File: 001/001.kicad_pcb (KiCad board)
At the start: 2 copper layers, 76.2 x 78.7 mm, 5 parts, among them SW1 SW_SPDT, U1 MF-Jalisco

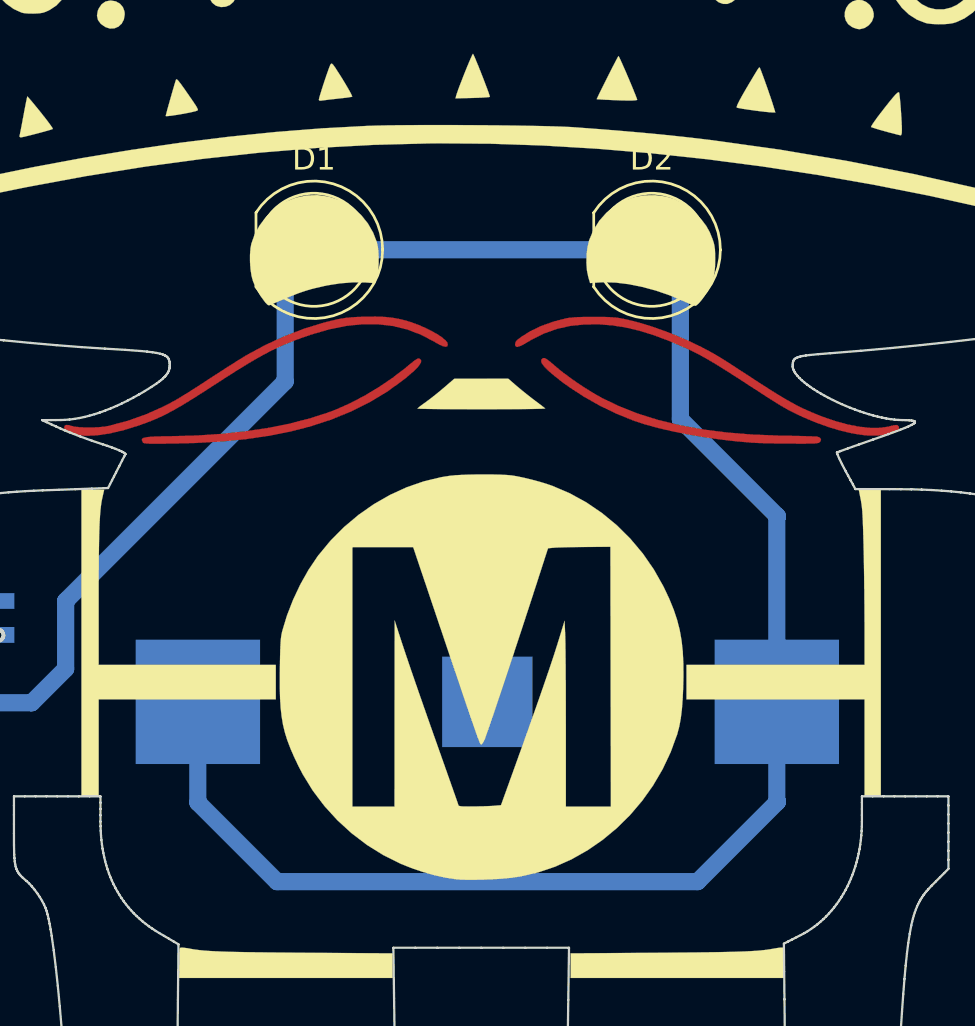
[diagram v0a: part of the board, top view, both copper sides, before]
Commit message: Add Battery Holder WA-BCMC and Straw Hat Led
Add Battery Holder WA-BCMC and Straw Hat Led
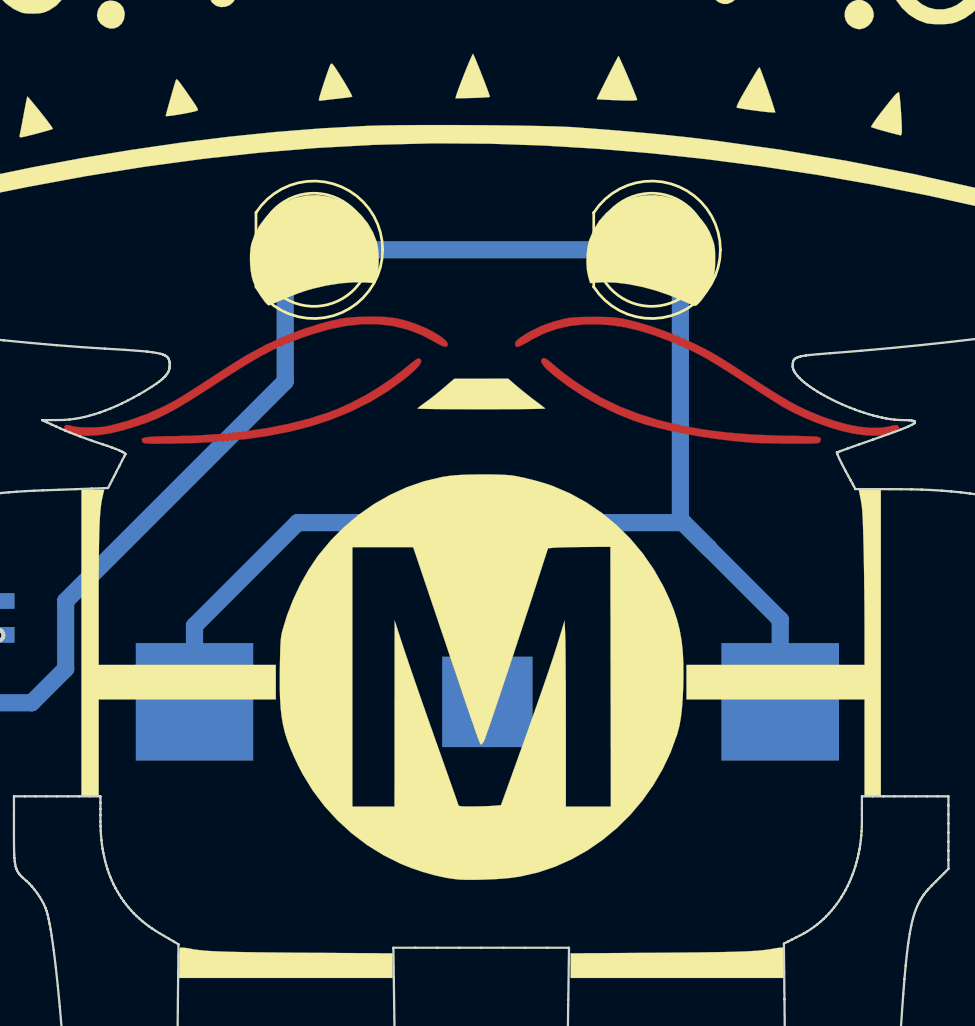
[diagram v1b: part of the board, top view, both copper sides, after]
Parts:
- BT1: footprint 001:S8211R -> 001:WA-BCMC
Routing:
- net +3V3: track 59.2 -> 50.3 mm
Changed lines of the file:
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@@
-(kicad_pcb (version 20171130) (host pcbnew 5.1.3-ffb9f22~84~ubuntu18.04.1)
+(kicad_pcb (version 20171130) (host pcbnew 5.1.4-e60b266~84~ubuntu18.04.1)
   (general
     (thickness 1.6002)
     (drawings 0)
-    (tracks 17)
+    (tracks 15)
     (zones 0)
     (modules 5)
@@
     (descr "LED, Round, FlatTop, diameter 5.0mm, 2 pins, http://www.kingbright.com/attachments/file/psearch/000/00/00/L-483GDT(Ver.15B).pdf")
     (tags "LED Round FlatTop diameter 5.0mm 2 pins")
-    (fp_text reference D1 (at 1.27 -4.01) (layer F.SilkS)
+    (fp_text reference D1 (at 1.27 -4.01) (layer F.Fab)
       (effects (font (size 1 1) (thickness 0.15)))
     )
@@
     (pad 2 thru_hole circle (at 2.54 0) (size 1.8 1.8) (drill 0.9) (layers *.Cu *.Mask)
       (net 1 "Net-(D1-Pad2)"))
-    (model ${KISYS3DMOD}/LED_THT.3dshapes/LED_D5.0mm_FlatTop.wrl
-      (at (xyz 0 0 0))
-      (scale (xyz 1 1 1))
-      (rotate (xyz 0 0 0))
+    (model "${KISYS3DMOD}/LED_THT.3dshapes/8mm 0.5w straw hat.STEP"
+      (offset (xyz 1.3 0 2.9))
+      (scale (xyz 0.5 0.7 0.5))
+      (rotate (xyz -90 0 180))
     )
   )
@@
     (descr "LED, Round, FlatTop, diameter 5.0mm, 2 pins, http://www.kingbright.com/attachments/file/psearch/000/00/00/L-483GDT(Ver.15B).pdf")
     (tags "LED Round FlatTop diameter 5.0mm 2 pins")
-    (fp_text reference D2 (at 1.27 -4.01) (layer F.SilkS)
+    (fp_text reference D2 (at 1.27 -4.01) (layer F.Fab)
       (effects (font (size 1 1) (thickness 0.15)))
     )
@@
     (pad 1 thru_hole rect (at 0 0) (size 1.8 1.8) (drill 0.9) (layers *.Cu *.Mask)
       (net 1 "Net-(D1-Pad2)"))
-    (model ${KISYS3DMOD}/LED_THT.3dshapes/LED_D5.0mm_FlatTop.wrl
-      (at (xyz 0 0 0))
-      (scale (xyz 1 1 1))
-      (rotate (xyz 0 0 0))
-    )
-  )
-  (module 001:S8211R (layer Back)
-    (at 137.3886 105.7148)
-    (fp_text reference BT1 (at 10.16 -12.446) (layer B.SilkS)
-      (effects (font (size 1 1) (thickness 0.15)) (justify mirror))
-    )
-    (fp_text value Battery_3V_Coin (at -9.398 10.16) (layer B.Fab)
-      (effects (font (size 1 1) (thickness 0.15)) (justify mirror))
-    )
-    (fp_line (start 12.8 9.1) (end 12.8 -10.9) (layer B.SilkS) (width 0.15))
-    (fp_line (start -12.8 9.1) (end 12.8 9.1) (layer B.SilkS) (width 0.15))
-    (fp_line (start -12.8 -10.9) (end -12.8 9.1) (layer B.SilkS) (width 0.15))
-    (fp_line (start 12.8 -10.9) (end -12.8 -10.9) (layer B.SilkS) (width 0.15))
-    (pad 1 smd rect (at 12.8 0) (size 5.5 5.5) (layers Back B.Paste B.Mask)
-      (net 2 +3V3))
-    (pad 1 smd rect (at -12.8 0) (size 5.5 5.5) (layers Back B.Paste B.Mask)
-      (net 2 +3V3))
-    (pad 2 smd rect (at 0 0) (size 4 4) (layers Back B.Paste B.Mask)
-      (net 3 GND))
-    (model /home/greynaga/Desktop/kicad/packages3d/Battery.3dshapes/s8211-46r.stp
-      (offset (xyz 0 6 4))
-      (scale (xyz 1 1 1))
-      (rotate (xyz 0 90 -90))
-    )
-    (model /home/greynaga/Desktop/kicad/packages3d/Battery.3dshapes/CR-2032-01.step
-      (offset (xyz 0 0 3))
-      (scale (xyz 1 1 1))
-      (rotate (xyz 90 0 0))
+    (model "${KISYS3DMOD}/LED_THT.3dshapes/8mm 0.5w straw hat.STEP"
+      (offset (xyz 1.3 0 2.9))
+      (scale (xyz 0.5 0.7 0.5))
+      (rotate (xyz -90 0 180))
     )
   )
@@
     )
   )
-  (via (at 115.7351 102.77094) (size 0.6858) (drill 0.3302) (layers Front Back) (net 3))
+  (module 001:WA-BCMC (layer Back)
+    (at 137.3886 105.7148)
+    (fp_text reference BT1 (at 10.16 -12.446) (layer B.Fab)
+      (effects (font (size 1 1) (thickness 0.15)) (justify mirror))
+    )
+    (fp_text value Battery_3V_Coin (at -9.398 10.16) (layer B.Fab)
+      (effects (font (size 1 1) (thickness 0.15)) (justify mirror))
+    )
+    (fp_line (start 12.8 -10.9) (end -12.8 -10.9) (layer B.Fab) (width 0.15))
+    (fp_line (start -12.8 -10.9) (end -12.8 9.1) (layer B.Fab) (width 0.15))
+    (fp_line (start -12.8 9.1) (end 12.8 9.1) (layer B.Fab) (width 0.15))
+    (fp_line (start 12.8 9.1) (end 12.8 -10.9) (layer B.Fab) (width 0.15))
+    (pad 2 smd rect (at 0 0) (size 4 4) (layers Back B.Paste B.Mask)
+      (net 3 GND))
+    (pad 1 smd rect (at -12.95 0) (size 5.2 5.2) (layers Back B.Paste B.Mask)
+      (net 2 +3V3))
+    (pad 1 smd rect (at 12.95 0) (size 5.2 5.2) (layers Back B.Paste B.Mask)
+      (net 2 +3V3))
+    (model ${KISYS3DMOD}/Battery.3dshapes/s8211-46r.stp
+      (offset (xyz 0 -6 4.1))
+      (scale (xyz 1 1 1))
+      (rotate (xyz 0 90 90))
+    )
+  )
   (segment (start 130.9878 85.725) (end 143.383 85.725) (width 0.762) (layer Back) (net 1))
-  (segment (start 145.923 93.218) (end 145.923 85.725) (width 0.762) (layer Back) (net 2))
-  (segment (start 150.214 97.509) (end 145.923 93.218) (width 0.762) (layer Back) (net 2))
-  (segment (start 150.1886 97.5344) (end 150.1886 105.7148) (width 0.762) (layer Back) (net 2))
-  (segment (start 150.214 97.509) (end 150.1886 97.5344) (width 0.762) (layer Back) (net 2))
-  (segment (start 124.5886 110.1666) (end 124.5886 105.7148) (width 0.762) (layer Back) (net 2))
-  (segment (start 128.087 113.665) (end 124.5886 110.1666) (width 0.762) (layer Back) (net 2))
-  (segment (start 150.214 110.136) (end 146.685 113.665) (width 0.762) (layer Back) (net 2))
-  (segment (start 146.685 113.665) (end 128.087 113.665) (width 0.762) (layer Back) (net 2))
-  (segment (start 150.1886 110.1106) (end 150.1886 105.7148) (width 0.762) (layer Back) (net 2))
-  (segment (start 150.214 110.136) (end 150.1886 110.1106) (width 0.762) (layer Back) (net 2))
+  (segment (start 150.3386 102.0786) (end 150.3386 105.7148) (width 0.762) (layer Back) (net 2))
+  (segment (start 147.193 98.933) (end 150.3386 102.0786) (width 0.762) (layer Back) (net 2))
+  (segment (start 145.923 97.663) (end 147.193 98.933) (width 0.762) (layer Back) (net 2))
+  (segment (start 145.923 85.725) (end 145.923 97.663) (width 0.762) (layer Back) (net 2))
+  (segment (start 146.05 97.79) (end 147.193 98.933) (width 0.762) (layer Back) (net 2))
+  (segment (start 129.0014 97.79) (end 146.05 97.79) (width 0.762) (layer Back) (net 2))
+  (segment (start 124.4386 105.7148) (end 124.4386 102.3528) (width 0.762) (layer Back) (net 2))
+  (segment (start 124.4386 102.3528) (end 129.0014 97.79) (width 0.762) (layer Back) (net 2))
+  (via (at 115.7351 102.77094) (size 0.6858) (drill 0.3302) (layers Front Back) (net 3))
   (segment (start 128.4478 91.54922) (end 128.4478 85.725) (width 0.762) (layer Back) (net 4))
   (segment (start 118.74246 101.25456) (end 128.4478 91.54922) (width 0.762) (layer Back) (net 4))
